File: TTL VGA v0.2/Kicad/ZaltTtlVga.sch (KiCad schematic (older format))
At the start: 2 parts

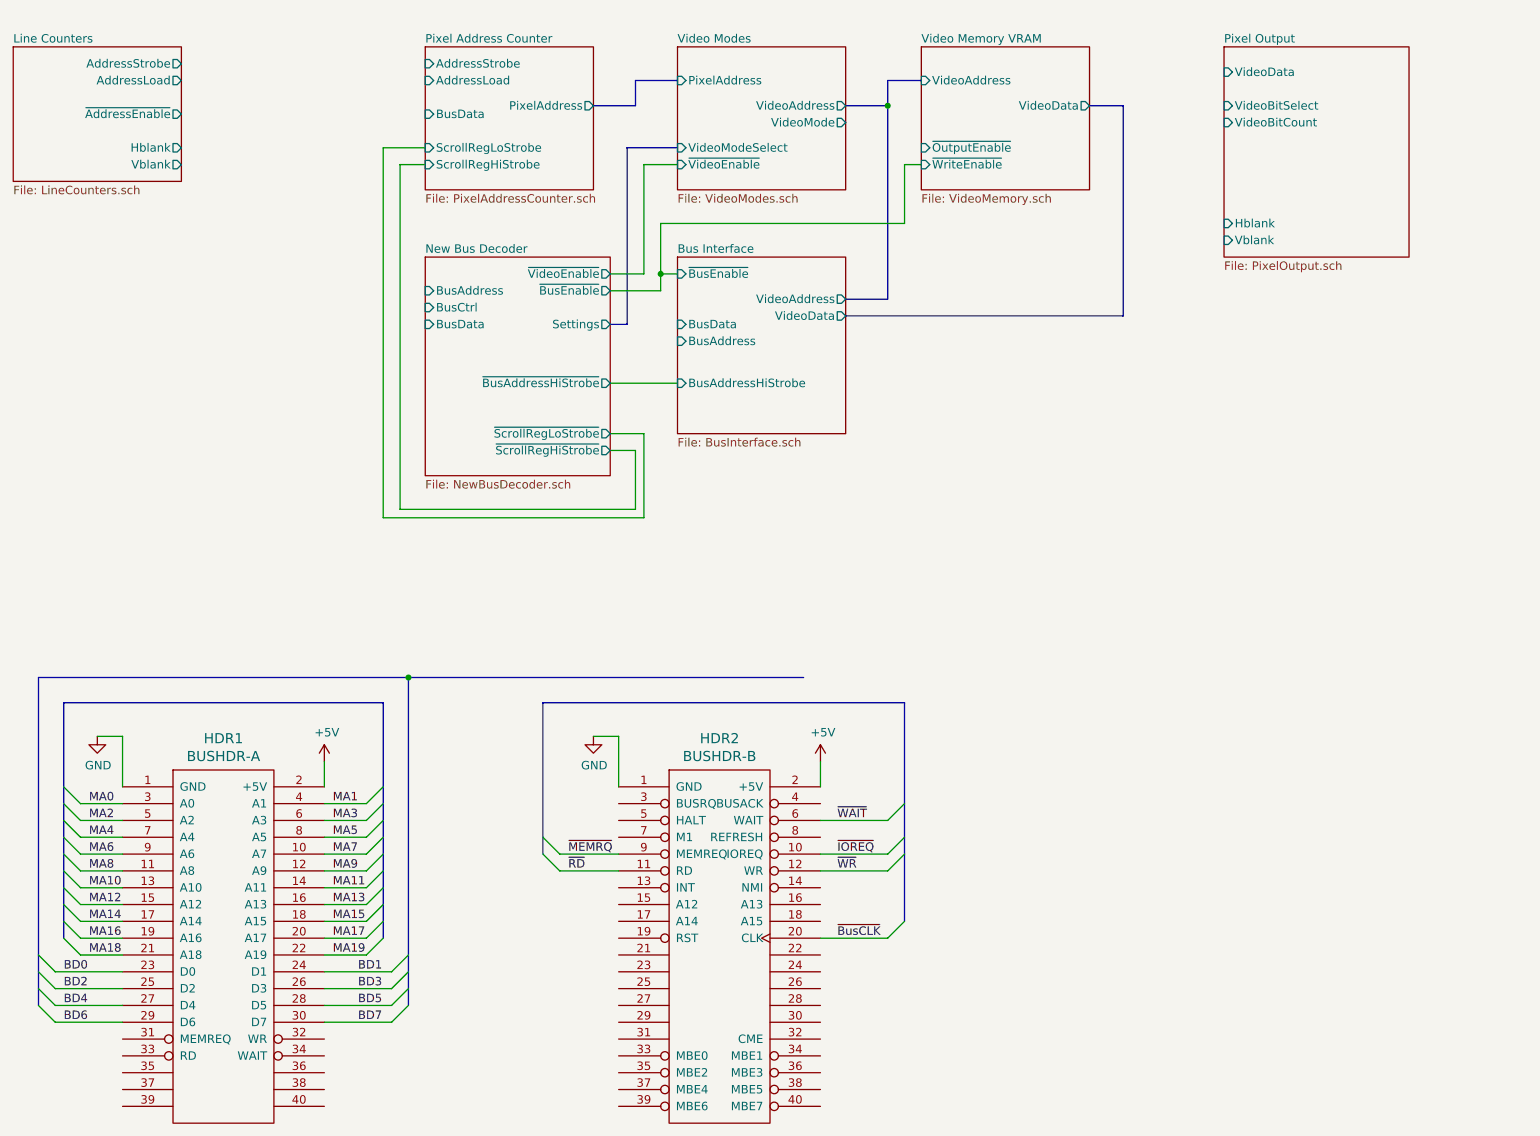
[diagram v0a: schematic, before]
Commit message: update kicad
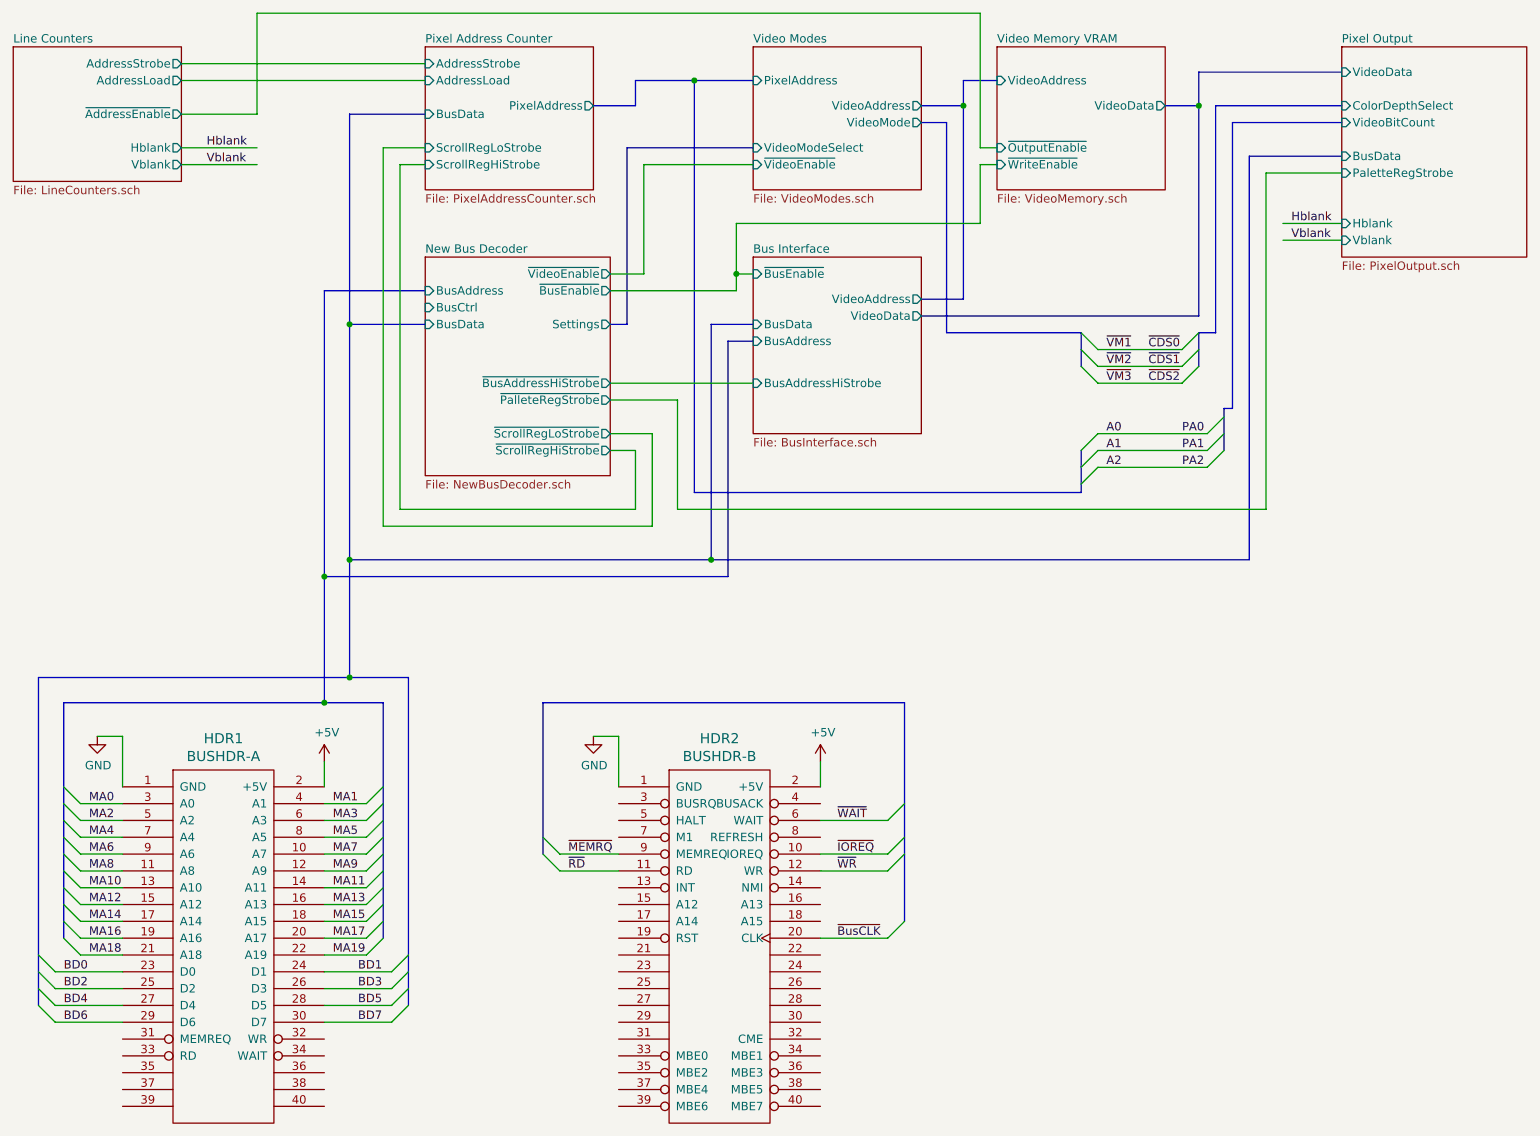
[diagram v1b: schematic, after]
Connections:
- net labels added: A0, A1, A2, Hblank, PA0, PA1, PA2, Vblank, ~CDS0, ~CDS1, ~CDS2, ~VM1, ~VM2, ~VM3
- wire segments 61 -> 83
